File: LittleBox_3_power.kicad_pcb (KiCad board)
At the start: 2 copper layers, 69 parts, among them P10 CONN_01X03, P13 CONN_01X03, P16 CONN_01X03, P17 CONN_01X03, P18 CONN_01X01, P19 CONN_01X03, P20 CONN_01X01, P21 CONN_01X01, P3 CONN_01X01, P4 CONN_01X01, P400IN+1 CONN_1, P400IN-1 CONN_1, P9 CONN_01X03, Q1 C3M0065090D, Q10 IPW6045CP, Q2 C3M0065090D, Q3 C3M0065090D, Q4 C3M0065090D, Q5 C3M0065090D, Q6 C3M0065090D, Q7 IPW6045CP, Q8 IPW6045CP, Q9 IPW6045CP, U18 ACS712, U19 ACS712, U21 ACS712, U23 ACS712, U5 ACS712, U6 ACS712

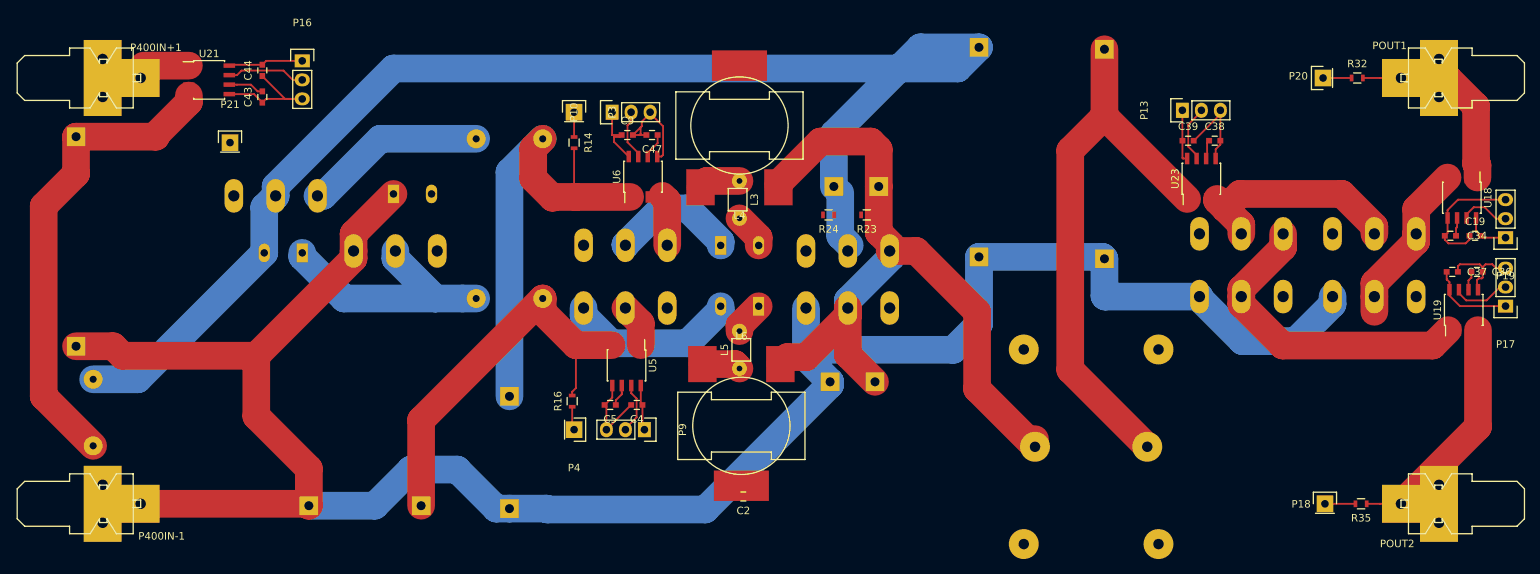
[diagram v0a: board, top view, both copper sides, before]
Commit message: Last mods
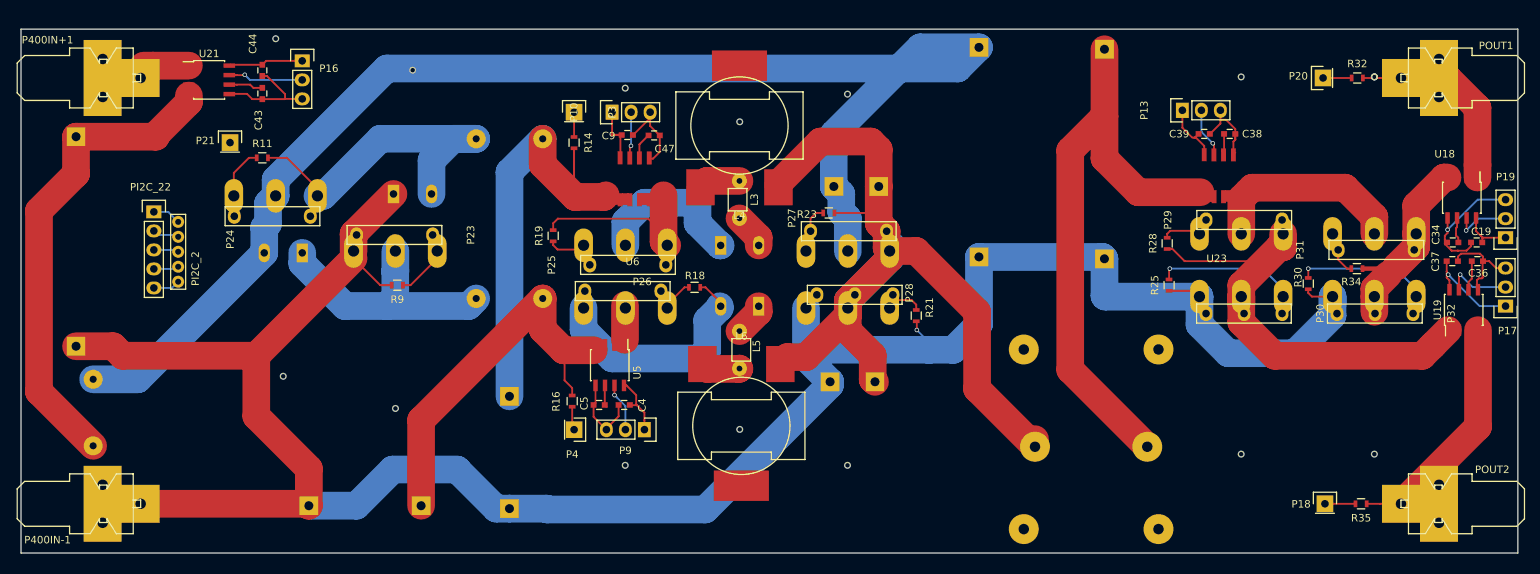
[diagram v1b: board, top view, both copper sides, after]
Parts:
- removed C2: 100n, Capacitors_SMD:C_0603
- removed R24: 1, Resistors_SMD:R_0603
- added ?: , inverter:hole_3mm, F.Cu at (110.5, 93.0)
- added ? (x2): , inverter:hole_3mm, F.Cu at (241.3, 48.7)
- added ?: , inverter:hole_3mm, F.Cu at (241.3, 99.1)
- added ?: , inverter:hole_3mm, F.Cu at (95.5, 88.7)
- added ?: , inverter:hole_3mm, F.Cu at (112.8, 47.8)
- added ?: , inverter:hole_3mm, F.Cu at (156.5, 95.8)
- added ?: , inverter:hole_3mm, F.Cu at (156.5, 54.7)
- added ?: , inverter:hole_3mm, F.Cu at (94.5, 43.6)
- added ?: , inverter:hole_3mm, F.Cu at (141.2, 100.6)
- added ?: , inverter:hole_3mm, F.Cu at (141.2, 50.2)
- added ?: , inverter:hole_3mm, F.Cu at (170.9, 100.6)
- added ?: , inverter:hole_3mm, F.Cu at (170.9, 51.0)
- added ?: , inverter:hole_3mm, F.Cu at (223.5, 48.7)
- added ?: , inverter:hole_3mm, F.Cu at (223.5, 99.1)
- added P23: CONN_01X02, inverter:Pin_Header_Straight_1x02_round, F.Cu at (115.5, 69.8)
- added P24: CONN_01X02, inverter:Pin_Header_Straight_1x02_round, F.Cu at (89.0, 67.3)
- added P25: CONN_01X02, inverter:Pin_Header_Straight_1x02_round, F.Cu at (136.5, 73.8)
- added P26: CONN_01X02, inverter:Pin_Header_Straight_1x02_round, F.Cu at (146.0, 77.3)
- added P27: CONN_01X02, inverter:Pin_Header_Straight_1x02_round, F.Cu at (166.0, 69.3)
- added P28: CONN_01X03, inverter:Pin_Header_Straight_1x03_round, F.Cu at (177.0, 77.8)
- added P29: CONN_01X02, inverter:Pin_Header_Straight_1x02_round, F.Cu at (218.8, 67.8)
- added P30: CONN_01X03, inverter:Pin_Header_Straight_1x03_round, F.Cu at (229.0, 80.3)
- added P31: CONN_01X02, inverter:Pin_Header_Straight_1x02_round, F.Cu at (236.5, 71.8)
- added P32: CONN_01X03, inverter:Pin_Header_Straight_1x03_round, F.Cu at (246.5, 80.3)
- added PI2C_2: CONN_01X05, inverter:Header_1x5_metric, F.Cu at (81.5, 72.1)
- added PI2C_22: CONN_01X05, Pin_Headers:Pin_Header_Straight_1x05, F.Cu at (78.2, 66.7)
- added R11: 1k, Resistors_SMD:R_0603, F.Cu at (92.7, 59.5)
- added R18: 1k, Resistors_SMD:R_0603, F.Cu at (150.5, 76.8)
- added R19: 1k, Resistors_SMD:R_0603, F.Cu at (131.6, 69.9)
- added R21: 1k, Resistors_SMD:R_0603, F.Cu at (180.1, 80.6)
- added R25: 1k, Resistors_SMD:R_0603, F.Cu at (213.9, 76.5)
- added R28: 1k, Resistors_SMD:R_0603, F.Cu at (213.6, 70.9)
- added R30: 1k, Resistors_SMD:R_0603, F.Cu at (232.5, 76.3)
- added R34: 1k, Resistors_SMD:R_0603, F.Cu at (239.0, 74.3)
- added R9: 1k, Resistors_SMD:R_0603, F.Cu at (110.7, 76.5)
- C4, C47, C5, C9: value 0.1u -> 100n
- U23, U6: footprint Housings_SOIC:SOIC-8_3.9x4.9mm_Pitch1.27mm -> inverter:ACS712
- moved R23 5.08 mm to (168.4, 66.9)
- moved U23 2.36 mm to (220.5, 61.9), turned to 0 degrees
- moved C39 2.34 mm to (218.6, 56.3)
- moved U5 2.24 mm to (139.1, 87.2)
- moved C38 2.20 mm to (222.0, 56.3)
- moved C4 1.68 mm to (141.1, 92.5)
- moved C5 1.47 mm to (137.7, 92.5)
- moved C36 1.44 mm to (255.1, 73.3)
- moved C37 1.44 mm to (251.7, 73.3)
- moved U6 1.15 mm to (142.5, 62.3), turned to 0 degrees
- moved C34 0.94 mm to (251.8, 70.8)
- moved C19 0.91 mm to (255.0, 70.8)
- moved C43 0.47 mm to (92.7, 50.9)
- moved C47 0.29 mm to (145.1, 56.5), turned to 0 degrees
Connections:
- net /M_I175 renamed Net-(P10-Pad2)
- net /M_I225 renamed Net-(P9-Pad2)
- net /M_IOUT2 renamed Net-(P17-Pad2)
- net /PB2 renamed Net-(P16-Pad2)
- net GND_P renamed GND_12
- net VCC3_A renamed VCC5_A
- P13 pad 2: /M_IOUT1 -> Net-(P13-Pad2)
- P19 pad 2: /M_IOUT1 -> Net-(P19-Pad2)
- U18 pad 7: /M_IOUT1 -> Net-(P19-Pad2)
- U23 pad 7: /M_IOUT1 -> Net-(P13-Pad2)
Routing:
- net GND_12: track 283.8 -> 308.9 mm, vias 0 -> 1
- net Net-(P30-Pad1): track 0.00 -> 21.1 mm, vias 0 -> 1
- net Net-(C13-Pad1): track 24.4 -> 45.3 mm
- net Net-(C32-Pad1): track 42.5 -> 63.3 mm
- net V175: track 6.87 -> 26.6 mm
- net /B1: track 102.4 -> 121.0 mm
- net Net-(P32-Pad1): track 0.00 -> 17.8 mm, vias 0 -> 1
- net /M_IOUT1: track 14.5 -> 0.00 mm
- net Net-(C21-Pad1): track 23.2 -> 32.3 mm
- net Net-(P19-Pad2): track 0.00 -> 8.26 mm, vias 0 -> 1
- net Net-(P23-Pad1): track 0.00 -> 7.06 mm
- net Net-(P13-Pad2): track 0.00 -> 7.00 mm, vias 0 -> 1
- net Net-(P24-Pad1): track 0.00 -> 6.96 mm
- net Net-(P27-Pad1): track 0.00 -> 6.59 mm
- net VCC5_A: track 50.5 -> 56.6 mm, vias 0 -> 1
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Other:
- board outline added: 200 x 70 mm
- net class 10A: clearance 0.3 -> 0.8
- net class 5A: clearance 0.3 -> 0.8
- net class Default: clearance 0.2 -> 0.25
- rule trace_clearance: 0.2 -> 0.25
